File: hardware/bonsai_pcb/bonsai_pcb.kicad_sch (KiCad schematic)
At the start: 5 parts, among them J1 Audio Amp Conn, J2 B+ Wire, J3 PH2.0 Battery Connector, SW1 BT1, U1 XIAO-ESP32-S3-SMD

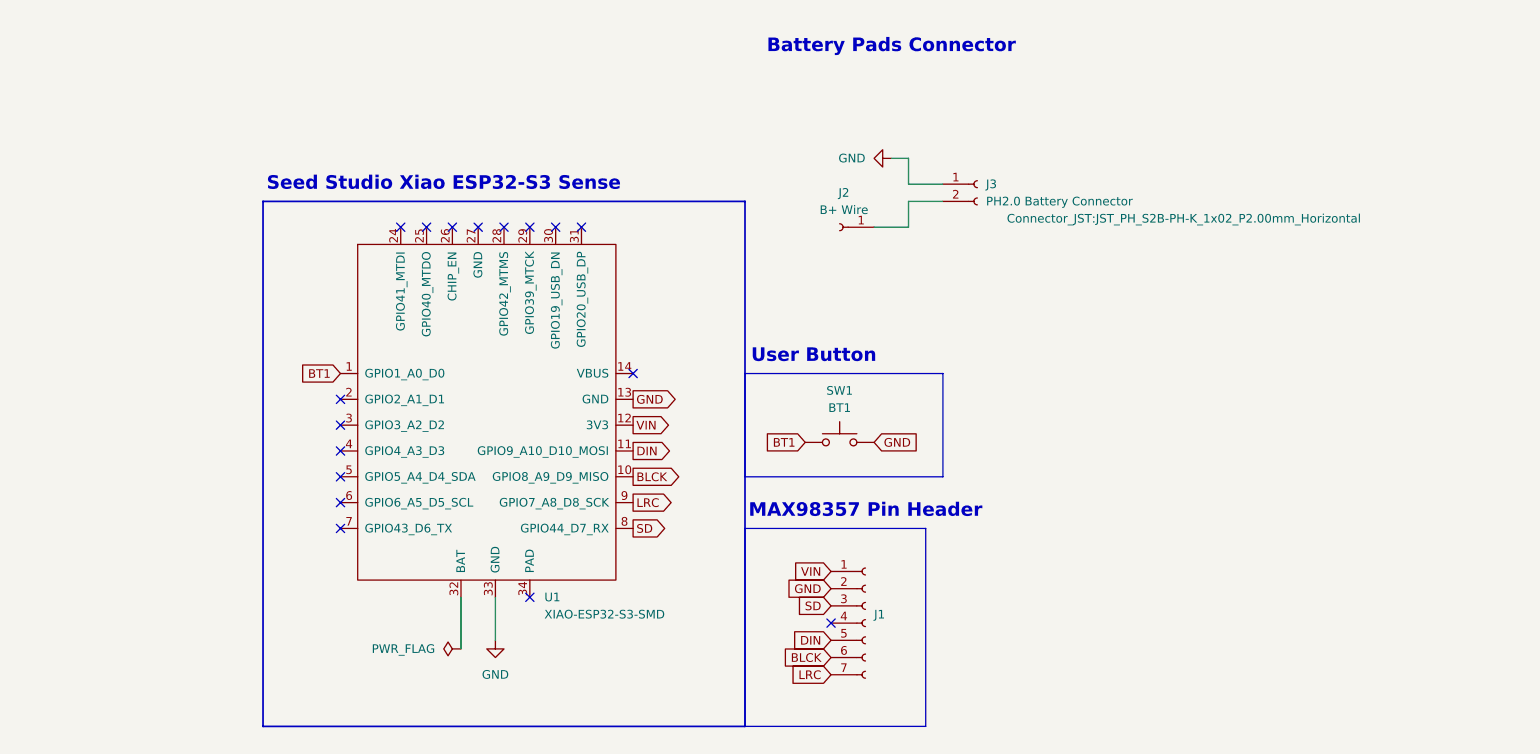
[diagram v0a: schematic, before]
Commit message: Update PCB, schematic, and STEP model
Co-Authored-By: Claude Sonnet 5 <noreply@anthropic.com>
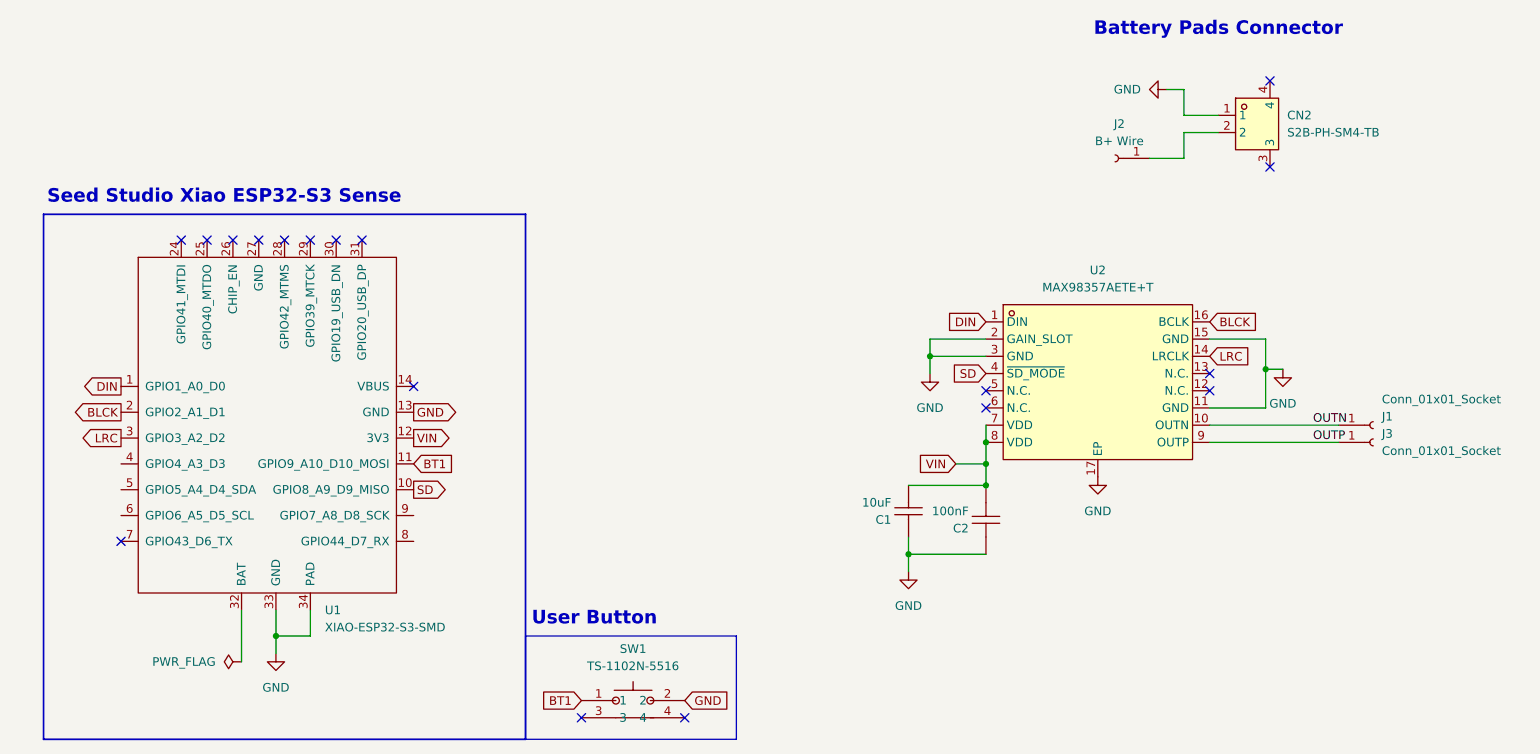
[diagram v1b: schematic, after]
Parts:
- removed J1: Audio Amp Conn, Connector_PinSocket_2.54mm:PinSocket_1x07_P2.54mm_Vertical, symbol Connector:Conn_01x07_Socket
- removed J3: PH2.0 Battery Connector, Connector_JST:JST_PH_S2B-PH-K_1x02_P2.00mm_Horizontal, symbol Connector:Conn_01x02_Socket
- removed SW1: BT1, Button_Switch_THT:SW_PUSH_6mm, symbol Switch:SW_Push
- added C1: 10uF, JLCPCB_Capacitors:C0402, symbol JLCPCB_Capacitors:CL05A106MQ5NUNC
- added C2: 100nF, JLCPCB_Capacitors:C0402, symbol JLCPCB_Capacitors:CL05B104KO5NNNC
- added CN2: S2B-PH-SM4-TB, JLCPCB_Connectors:CONN-SMD_P2.00_S2B-PH-SM4-TB-LF-SN, symbol JLCPCB_Connectors:S2B-PH-SM4-TB
- added J1, J3: Conn_01x01_Socket, Connector_Wire:SolderWirePad_1x01_SMD_2x4mm, symbol Connector:Conn_01x01_Socket
- added SW1: TS-1102N-5516, JLCPCB_Switches:SW-TH_TS-1102N-5516, symbol JLCPCB_Switches:TS-1102N-5516
- added U2: MAX98357AETE+T, JLCPCB_Amplifiers:TQFN-16_L3.0-W3.0-P0.50-BL-EP1.5, symbol JLCPCB_Amplifiers:MAX98357AETE+T
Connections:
- net BLCK: now also U1.2 (GPIO2_A1_D1), U2.16 (BCLK); no longer U1.10 (GPIO8_A9_D9_MISO)
- net BT1: now also U1.11 (GPIO9_A10_D10_MOSI), SW1.1; no longer U1.1 (GPIO1_A0_D0)
- net DIN: now also U1.1 (GPIO1_A0_D0), U2.1 (DIN); no longer U1.11 (GPIO9_A10_D10_MOSI)
- net GND: now also U1.34 (PAD), C1.2, C2.2, CN2.1, SW1.2, U2.11 (GND), U2.15 (GND), U2.17 (EP), U2.2 (GAIN_SLOT), U2.3 (GND)
- net LRC: now also U1.3 (GPIO3_A2_D2), U2.14 (LRCLK); no longer U1.9 (GPIO7_A8_D8_SCK)
- net SD: now also U1.10 (GPIO8_A9_D9_MISO), U2.4 (~{SD_MODE}); no longer U1.8 (GPIO44_D7_RX)
- net VIN: now also C1.1, C2.1, U2.7 (VDD), U2.8 (VDD)
- net at J2.1 (Pin_1): now also CN2.2
- new net OUTN: J1.1 (Pin_1), U2.10 (OUTN)
- new net OUTP: J3.1 (Pin_1), U2.9 (OUTP)
- no-connect marks 17 -> 18
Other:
- note removed: "MAX98357 Pin Header"
- moved on the sheet: J2, U1
